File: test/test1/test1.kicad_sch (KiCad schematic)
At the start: 2 parts, among them U1 module_mpu6050, U2 mini_esp32

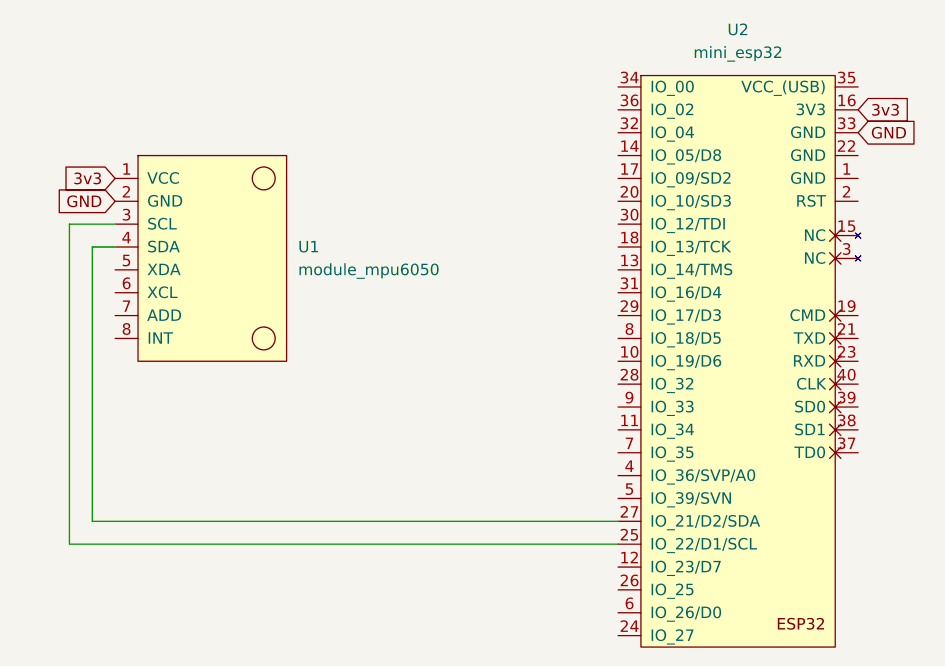
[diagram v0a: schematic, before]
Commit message: tété
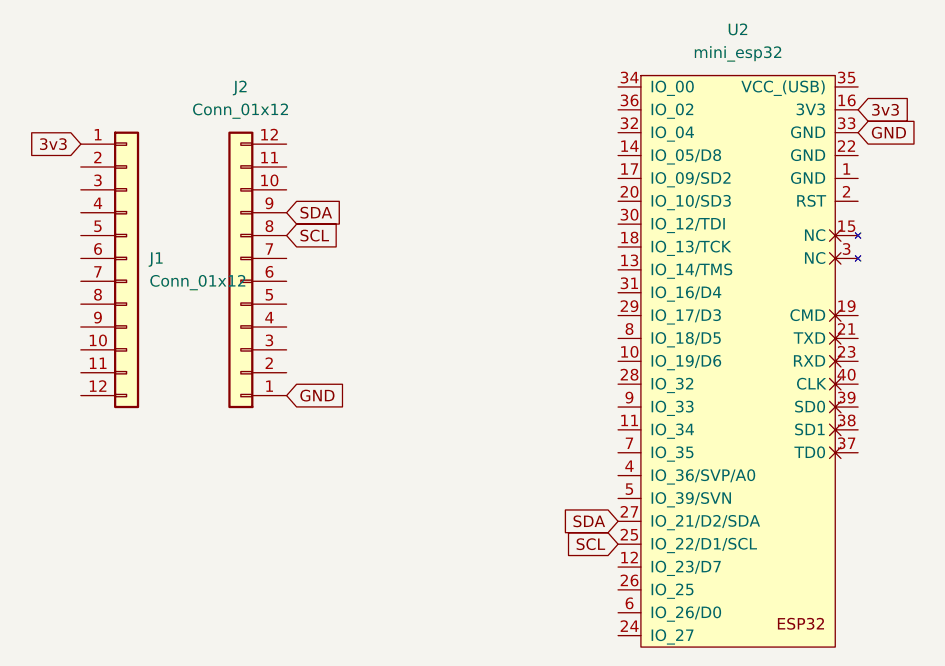
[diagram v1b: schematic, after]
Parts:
- removed U1: module_mpu6050, usini_sensors:module_mpu6050, symbol usini_sensors:module_mpu6050
- added J1, J2: Conn_01x12, Connector_PinSocket_2.54mm:PinSocket_1x11_P2.54mm_Vertical, symbol Connector_Generic:Conn_01x12
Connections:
- net 3v3: now also J1.1 (Pin_1)
- net GND: now also J2.1 (Pin_1)
- net SCL: now reaches U2.25 (IO_22/D1/SCL)
- net SCL: now also J2.8 (Pin_8)
- net SDA: now reaches U2.27 (IO_21/D2/SDA)
- net SDA: now also J2.9 (Pin_9)
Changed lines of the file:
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@@
 (kicad_sch (version 20211123) (generator eeschema)
   (paper "A4")
-  (wire (pts (xy 87.63 55.88) (xy 85.09 55.88))
-    (stroke (width 0) (type default) (color 0 0 0 0))
-  )
-  (wire (pts (xy 82.55 88.9) (xy 82.55 53.34))
-    (stroke (width 0) (type default) (color 0 0 0 0))
-  )
-  (wire (pts (xy 85.09 86.36) (xy 143.51 86.36))
-    (stroke (width 0) (type default) (color 0 0 0 0))
-  )
-  (wire (pts (xy 82.55 53.34) (xy 87.63 53.34))
-    (stroke (width 0) (type default) (color 0 0 0 0))
-  )
-  (wire (pts (xy 85.09 55.88) (xy 85.09 86.36))
-    (stroke (width 0) (type default) (color 0 0 0 0))
-  )
-  (wire (pts (xy 143.51 88.9) (xy 82.55 88.9))
-    (stroke (width 0) (type default) (color 0 0 0 0))
-  )
-  (global_label "3v3" (shape input) (at 87.63 48.26 180) (fields_autoplaced)
-    (effects (font (size 1.27 1.27)) (justify right))
-    (property "Intersheet References" "${INTERSHEET_REFS}" (id 0) (at 81.8302 48.3394 0)
-      (effects (font (size 1.27 1.27)) (justify right) hide)
+  (global_label "SCL" (shape input) (at 106.68 54.61 0) (fields_autoplaced)
+    (effects (font (size 1.27 1.27)) (justify left))
+    (property "Intersheet References" "${INTERSHEET_REFS}" (id 0) (at 112.6007 54.5306 0)
+      (effects (font (size 1.27 1.27)) (justify left) hide)
     )
   )
@@
     )
   )
+  (global_label "GND" (shape input) (at 106.68 72.39 0) (fields_autoplaced)
+    (effects (font (size 1.27 1.27)) (justify left))
+    (property "Intersheet References" "${INTERSHEET_REFS}" (id 0) (at 112.9636 72.3106 0)
+      (effects (font (size 1.27 1.27)) (justify left) hide)
+    )
+  )
+  (global_label "SCL" (shape input) (at 143.51 88.9 180) (fields_autoplaced)
+    (effects (font (size 1.27 1.27)) (justify right))
+    (property "Intersheet References" "${INTERSHEET_REFS}" (id 0) (at 137.5893 88.9794 0)
+      (effects (font (size 1.27 1.27)) (justify right) hide)
+    )
+  )
   (global_label "GND" (shape input) (at 170.18 43.18 0) (fields_autoplaced)
     (effects (font (size 1.27 1.27)) (justify left))
@@
     )
   )
-  (global_label "GND" (shape input) (at 87.63 50.8 180) (fields_autoplaced)
+  (global_label "SDA" (shape input) (at 106.68 52.07 0) (fields_autoplaced)
+    (effects (font (size 1.27 1.27)) (justify left))
+    (property "Intersheet References" "${INTERSHEET_REFS}" (id 0) (at 112.6612 51.9906 0)
+      (effects (font (size 1.27 1.27)) (justify left) hide)
+    )
+  )
+  (global_label "3v3" (shape input) (at 83.82 44.45 180) (fields_autoplaced)
     (effects (font (size 1.27 1.27)) (justify right))
-    (property "Intersheet References" "${INTERSHEET_REFS}" (id 0) (at 81.3464 50.8794 0)
+    (property "Intersheet References" "${INTERSHEET_REFS}" (id 0) (at 78.0202 44.5294 0)
       (effects (font (size 1.27 1.27)) (justify right) hide)
     )
   )
-  (symbol (lib_id "usini_sensors:module_mpu6050") (at 87.63 66.04 0) (unit 1)
+  (global_label "SDA" (shape input) (at 143.51 86.36 180) (fields_autoplaced)
+    (effects (font (size 1.27 1.27)) (justify right))
+    (property "Intersheet References" "${INTERSHEET_REFS}" (id 0) (at 137.5288 86.4394 0)
+      (effects (font (size 1.27 1.27)) (justify right) hide)
+    )
+  )
+  (symbol (lib_id "Connector_Generic:Conn_01x12") (at 88.9 57.15 0) (unit 1)
     (in_bom yes) (on_board yes) (fields_autoplaced)
-    (property "Reference" "U1" (id 0) (at 107.95 55.8799 0)
+    (property "Reference" "J1" (id 0) (at 91.44 57.1499 0)
       (effects (font (size 1.27 1.27)) (justify left))
     )
-    (property "Value" "module_mpu6050" (id 1) (at 107.95 58.4199 0)
+    (property "Value" "Conn_01x12" (id 1) (at 91.44 59.6899 0)
       (effects (font (size 1.27 1.27)) (justify left))
     )
-    (property "Footprint" "usini_sensors:module_mpu6050" (id 2) (at 99.06 72.39 0)
+    (property "Footprint" "Connector_PinSocket_2.54mm:PinSocket_1x11_P2.54mm_Vertical" (id 2) (at 88.9 57.15 0)
       (effects (font (size 1.27 1.27)) hide)
     )
-    (property "Datasheet" "" (id 3) (at 87.63 59.69 0)
+    (property "Datasheet" "~" (id 3) (at 88.9 57.15 0)
       (effects (font (size 1.27 1.27)) hide)
     )
     (pin "1")
+    (pin "10")
+    (pin "11")
+    (pin "12")
     (pin "2")
     (pin "3")
@@
     (pin "7")
     (pin "8")
+    (pin "9")
   )
   (symbol (lib_id "ESP32_mini:mini_esp32") (at 156.21 35.56 0) (unit 1)
@@
     (pin "9")
   )
+  (symbol (lib_id "Connector_Generic:Conn_01x12") (at 101.6 59.69 180) (unit 1)
+    (in_bom yes) (on_board yes) (fields_autoplaced)
+    (property "Reference" "J2" (id 0) (at 101.6 38.1 0))
+    (property "Value" "Conn_01x12" (id 1) (at 101.6 40.64 0))
+    (property "Footprint" "Connector_PinSocket_2.54mm:PinSocket_1x11_P2.54mm_Vertical" (id 2) (at 101.6 59.69 0)
+      (effects (font (size 1.27 1.27)) hide)
+    )
+    (property "Datasheet" "~" (id 3) (at 101.6 59.69 0)
+      (effects (font (size 1.27 1.27)) hide)
+    )
+    (pin "1")
+    (pin "10")
+    (pin "11")
+    (pin "12")
+    (pin "2")
+    (pin "3")
+    (pin "4")
+    (pin "5")
+    (pin "6")
+    (pin "7")
+    (pin "8")
+    (pin "9")
+  )
   (sheet_instances
     (path "/" (page "1"))
   )
   (symbol_instances
-    (path "/2c91c904-4d5a-4403-a61c-768bb93a8c7e"
-      (reference "U1") (unit 1) (value "module_mpu6050") (footprint "usini_sensors:module_mpu6050")
+    (path "/564d691c-9f25-47d5-a421-d002b9a03357"
+      (reference "J1") (unit 1) (value "Conn_01x12") (footprint "Connector_PinSocket_2.54mm:PinSocket_1x11_P2.54mm_Vertical")
+    )
+    (path "/95489415-dcfc-4ecb-91af-091a7dad7566"
+      (reference "J2") (unit 1) (value "Conn_01x12") (footprint "Connector_PinSocket_2.54mm:PinSocket_1x11_P2.54mm_Vertical")
     )
     (path "/776caef5-77e8-479d-9002-efa59d947083"
